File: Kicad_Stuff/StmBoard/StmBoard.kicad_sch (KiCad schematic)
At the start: 2 parts, among them U1 STM32G031K8Tx, U2 LIS3DH

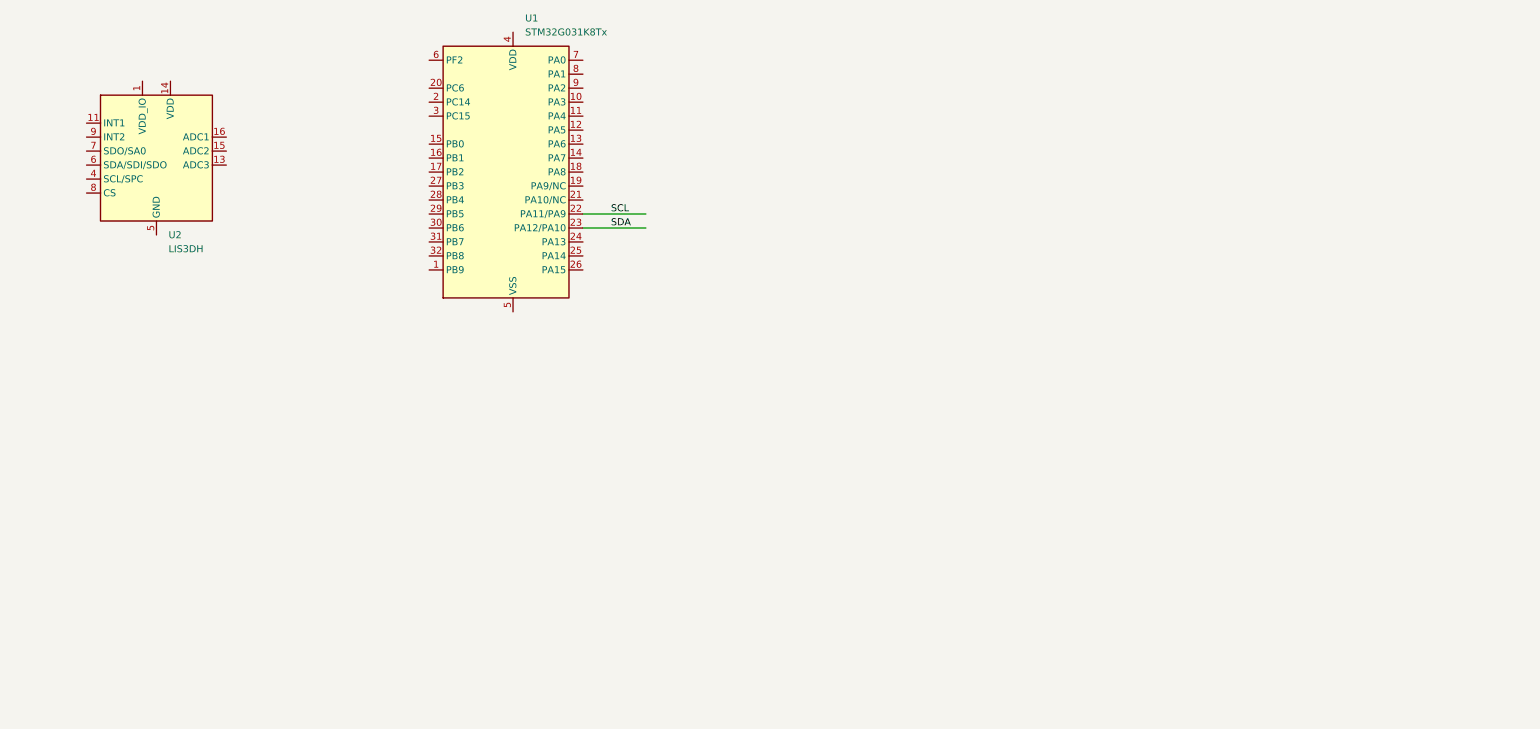
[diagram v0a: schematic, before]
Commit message: quick commit
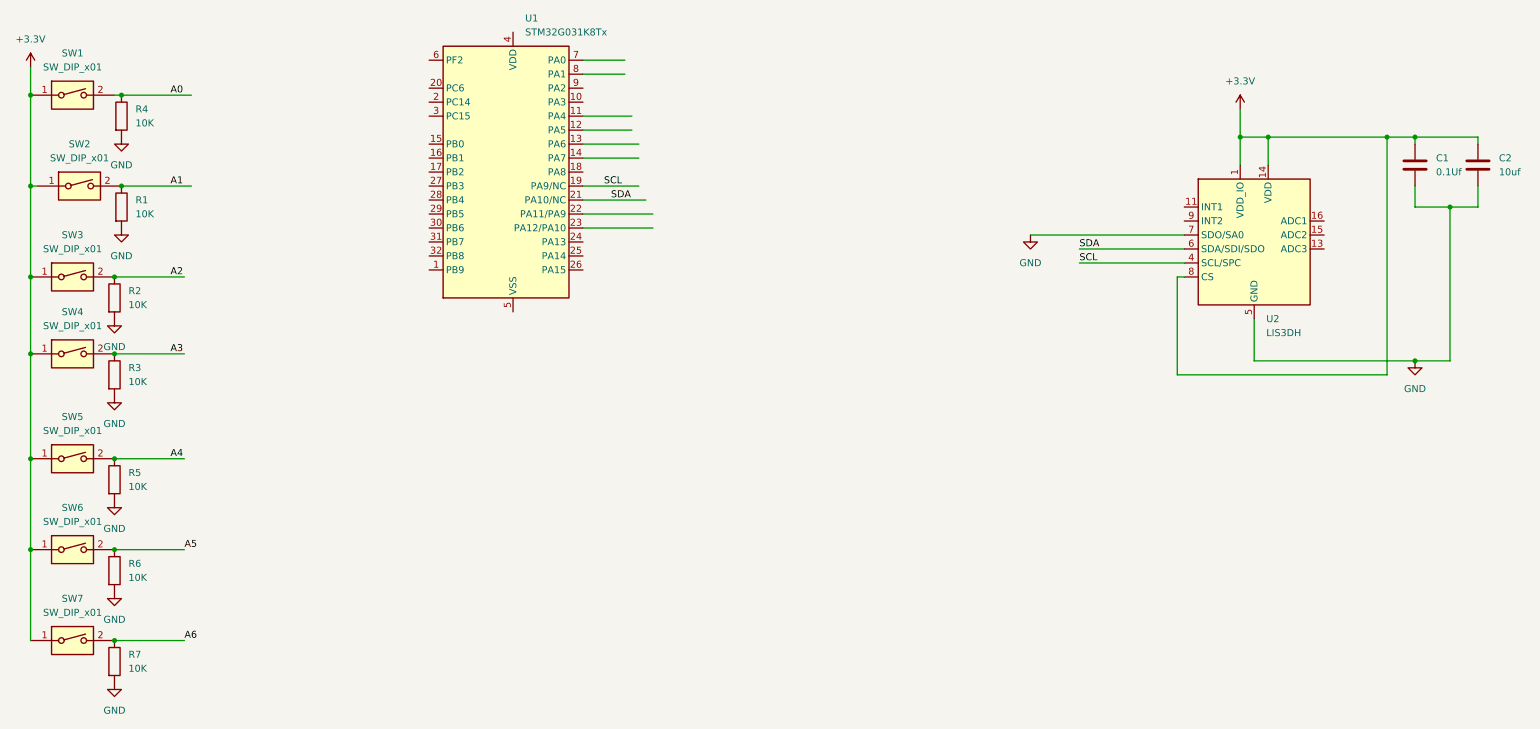
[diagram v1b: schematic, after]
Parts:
- added C1: 0.1Uf, symbol Device:C
- added C2: 10uf, symbol Device:C
- added R1, R2, R3, R4, R5, R6, R7: 10K, symbol Device:R
- added SW1, SW2, SW3, SW4, SW5, SW6, SW7: SW_DIP_x01, symbol Switch:SW_DIP_x01
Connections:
- net SCL: now also U1.19 (PA9/NC), U2.4 (SCL/SPC); no longer U1.22 (PA11/PA9)
- net SDA: now also U1.21 (PA10/NC), U2.6 (SDA/SDI/SDO); no longer U1.23 (PA12/PA10)
- net +3.3V: now reaches U2.1 (VDD_IO)
- net +3.3V: now also U2.14 (VDD), U2.8 (CS), C1.1, C2.1, SW1.1, SW2.1, SW3.1, SW4.1, SW5.1, SW6.1, SW7.1
- net GND: now reaches U2.10 (GND), U2.12 (GND), U2.5 (GND)
- net GND: now also U2.7 (SDO/SA0), C1.2, C2.2, R1.2, R2.2, R3.2, R4.2, R5.2, R6.2, R7.2
- new net A0: R4.1, SW1.2
- new net A1: R1.1, SW2.2
- new net A2: R2.1, SW3.2
- new net A3: R3.1, SW4.2
- new net A4: R5.1, SW5.2
- new net A5: R6.1, SW6.2
- new net A6: R7.1, SW7.2
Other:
- moved on the sheet: U2
